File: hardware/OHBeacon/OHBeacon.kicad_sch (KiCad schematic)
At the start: 10 parts, among them J1 Conn_01x04_Socket, SW1 SW_Push, U1 ESP32-C3-WROOM-02

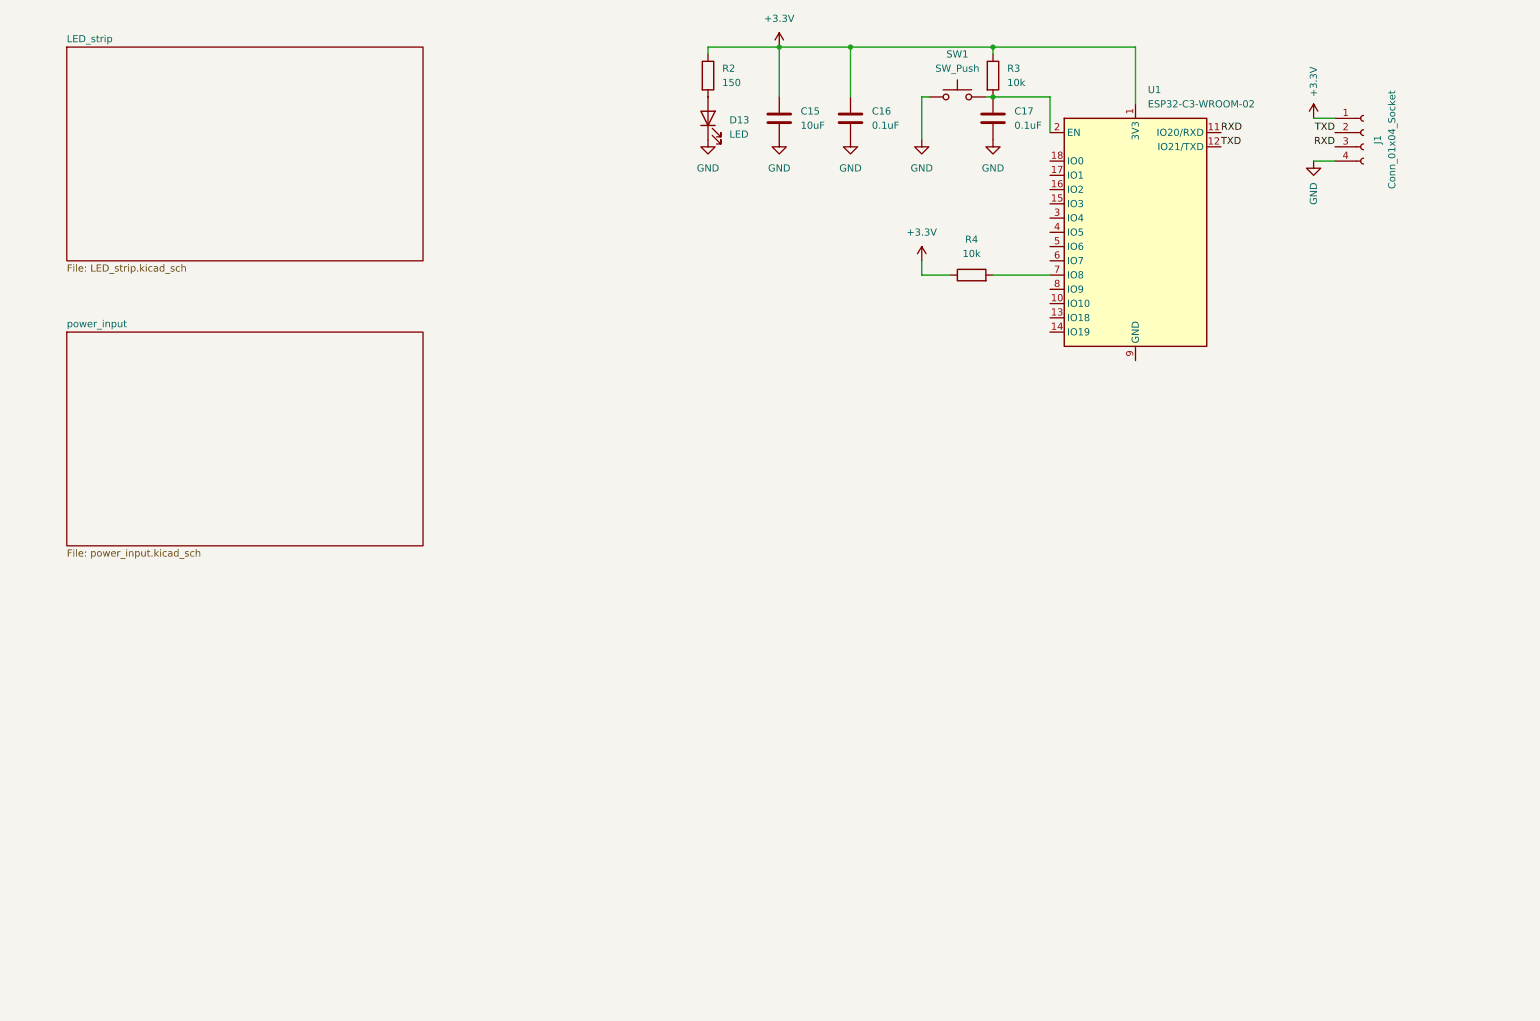
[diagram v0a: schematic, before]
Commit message: new sch
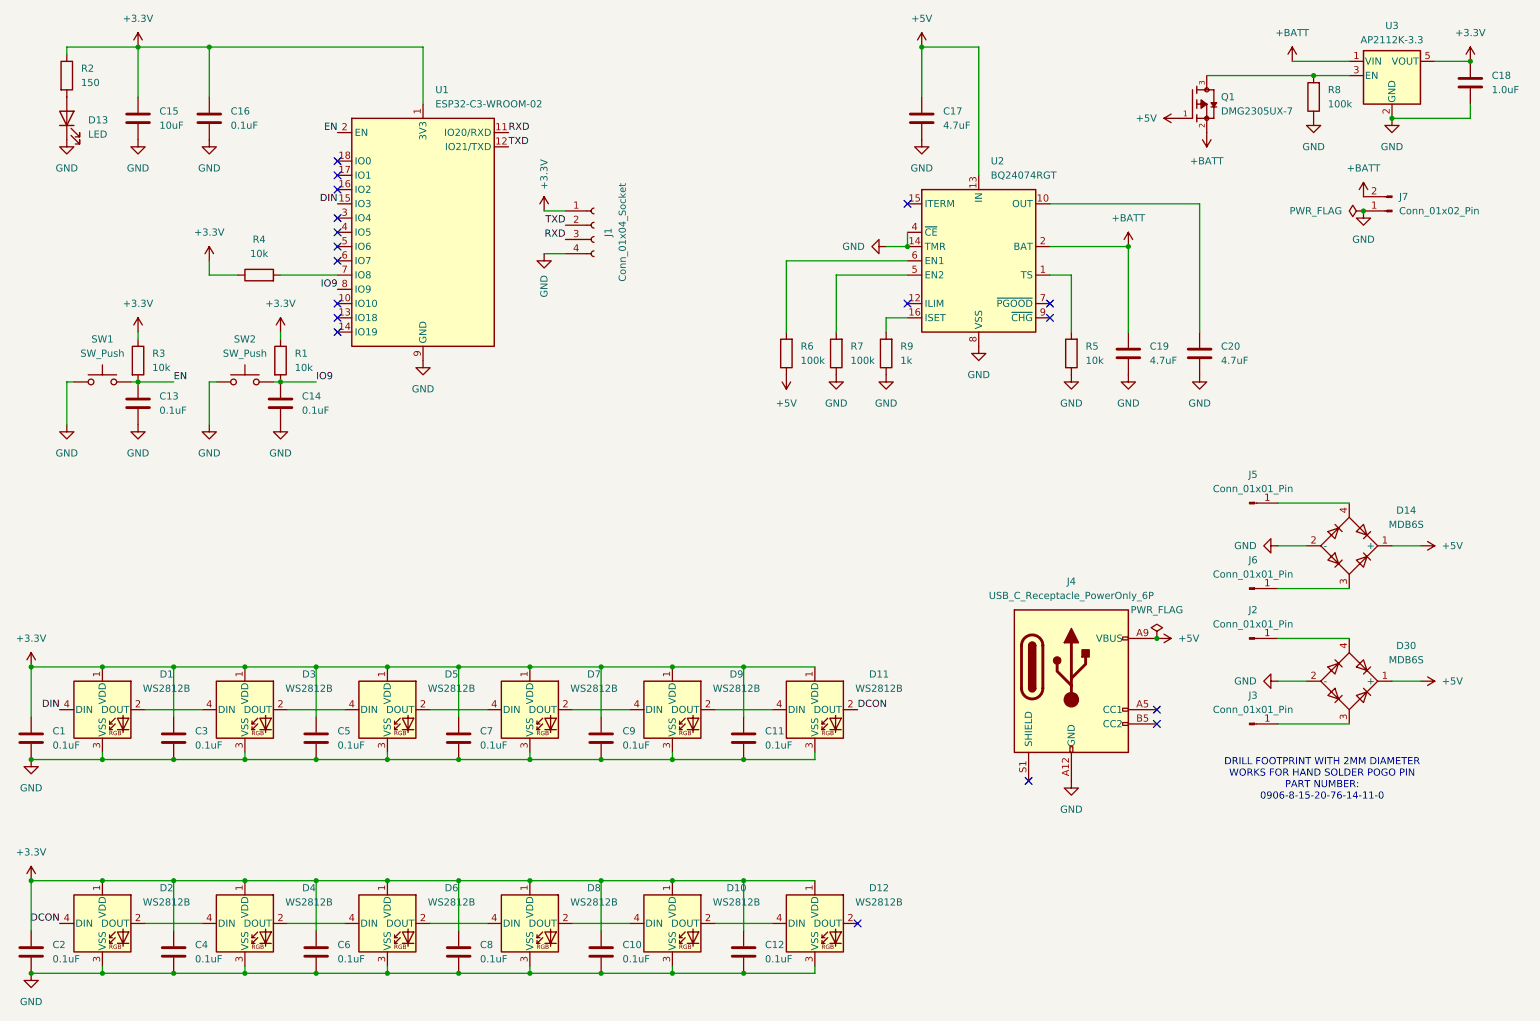
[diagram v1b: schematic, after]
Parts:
- added C1, C10, C11, C12, C13, C14, C2, C3, C4, C5, C6, C7, C8, C9: 0.1uF, Capacitor_SMD:C_0603_1608Metric, symbol Device:C
- added C18: 1.0uF, Capacitor_SMD:C_0603_1608Metric, symbol Device:C
- added C19, C20: 4.7uF, Capacitor_SMD:C_0603_1608Metric, symbol Device:C
- added D1, D10, D11, D12, D2, D3, D4, D5, D6, D7, D8, D9: WS2812B, LED_SMD:LED_WS2812B_PLCC4_5.0x5.0mm_P3.2mm, symbol LED:WS2812B
- added D14, D30: MDB6S, Package_SO:TSSOP-4_4.4x5mm_P4mm, symbol Diode_Bridge:MDB6S
- added J2, J3, J5, J6: Conn_01x01_Pin, Connector_Wire:SolderWire-2sqmm_1x01_D2mm_OD3.9mm, symbol Connector:Conn_01x01_Pin
- added J4: USB_C_Receptacle_PowerOnly_6P, Connector_USB:USB_C_Receptacle_GCT_USB4135-GF-A_6P_TopMnt_Horizontal, symbol Connector:USB_C_Receptacle_PowerOnly_6P
- added J7: Conn_01x02_Pin, Connector_PinSocket_2.54mm:PinSocket_1x02_P2.54mm_Vertical, symbol Connector:Conn_01x02_Pin
- added Q1: DMG2305UX-7, DMG2305UX-7:SOT91P240X110-3N_DMG2305UX-7, symbol DMG2305UX-7:DMG2305UX-7
- added R1, R5: 10k, Resistor_SMD:R_0603_1608Metric, symbol Device:R
- added R6, R7, R8: 100k, Resistor_SMD:R_0603_1608Metric, symbol Device:R
- added R9: 1k, Resistor_SMD:R_0603_1608Metric, symbol Device:R
- added SW2: SW_Push, Button_Switch_THT:SW_PUSH_6mm, symbol Switch:SW_Push
- added U2: BQ24074RGT, Package_DFN_QFN:VQFN-16-1EP_3x3mm_P0.5mm_EP1.6x1.6mm, symbol Battery_Management:BQ24074RGT
- added U3: AP2112K-3.3, Package_TO_SOT_SMD:SOT-23-5, symbol Regulator_Linear:AP2112K-3.3
- C17: value 0.1uF -> 4.7uF
- SW1: footprint Buttons_Switches_THT.pretty-master:SW_PUSH_6mm -> Button_Switch_THT:SW_PUSH_6mm
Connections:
- net +3.3V: now also C1.1, C10.1, C11.1, C12.1, C18.1, C2.1, C3.1, C4.1, C5.1, C6.1, C7.1, C8.1, C9.1, D1.1 (VDD), D10.1 (VDD), D11.1 (VDD), D12.1 (VDD), D2.1 (VDD), D3.1 (VDD), D4.1 (VDD), D5.1 (VDD), D6.1 (VDD), D7.1 (VDD), D8.1 (VDD), D9.1 (VDD), R1.1, U3.5 (VOUT)
- net GND: now also U1.19 (GND), U1.9 (GND), C1.2, C10.2, C11.2, C12.2, C13.2, C14.2, C18.2, C19.2, C2.2, C20.2, C3.2, C4.2, C5.2, C6.2, C7.2, C8.2, C9.2, D1.3 (VSS), D10.3 (VSS), D11.3 (VSS), D12.3 (VSS), D14.2 (-), D2.3 (VSS), D3.3 (VSS), D30.2 (-), D4.3 (VSS), D5.3 (VSS), D6.3 (VSS), D7.3 (VSS), D8.3 (VSS), D9.3 (VSS), J4.A12 (GND), J4.B12 (GND), J7.1 (Pin_1), R5.1, R7.1, R8.1, R9.1, SW2.1, U2.14 (TMR), U2.17 (VSS), U2.4 (~{CE}), U2.8 (VSS), U3.2 (GND)
- net EN: now reaches R3.2, SW1.2, U1.2 (EN)
- net EN: now also C13.1; no longer C17.1
- net DIN: now reaches U1.15 (IO3)
- net DIN: now also D1.4 (DIN)
- net IO9: now reaches U1.8 (IO9)
- net IO9: now also C14.1, R1.2, SW2.2
- new net: C20.1, U2.10 (OUT), U2.11 (OUT)
- new net: Q1.3, R8.2, U3.3 (EN)
- new net: R5.2, U2.1 (TS)
- new net: R9.2, U2.16 (ISET)
- new net: R7.2, U2.5 (EN2)
- new net: R6.2, U2.6 (EN1)
- new net: D30.3, J3.1 (Pin_1)
- new net: D30.4, J2.1 (Pin_1)
- new net: D10.2 (DOUT), D12.4 (DIN)
- new net: D5.2 (DOUT), D7.4 (DIN)
- new net: D3.2 (DOUT), D5.4 (DIN)
- new net: D1.2 (DOUT), D3.4 (DIN)
- new net: D4.2 (DOUT), D6.4 (DIN)
- new net: D2.2 (DOUT), D4.4 (DIN)
- new net: D11.4 (DIN), D9.2 (DOUT)
- new net: D7.2 (DOUT), D9.4 (DIN)
- new net: D10.4 (DIN), D8.2 (DOUT)
- new net: D6.2 (DOUT), D8.4 (DIN)
- new net: D14.3, J6.1 (Pin_1)
- new net: D14.4, J5.1 (Pin_1)
- new net +5V: C17.1, D14.1 (+), D30.1 (+), J4.A9 (VBUS), J4.B9 (VBUS), Q1.1, R6.1, U2.13 (IN)
- new net +BATT: C19.1, J7.2 (Pin_2), Q1.2, U2.2 (BAT), U2.3 (BAT), U3.1 (VIN)
- new net DCON: D11.2 (DOUT), D2.4 (DIN)
- no-connect marks 0 -> 18
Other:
- removed sheet LED_strip
- removed sheet power_input
- note added: "DRILL FOOTPRINT WITH 2MM DIAMETER WORKS FOR HAND SOLDER POGO PIN PART NUMBER: 0906-8-15-20-76-14-11-0"
- moved on the sheet: C15, C16, J1, R2, R4, U1
